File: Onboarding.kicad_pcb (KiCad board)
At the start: 2 copper layers, 40.5 x 26.5 mm, 21 parts, among them J1 Conn_01x02_Female, J2 Conn_01x02_Male, J3 Conn_01x02, J4 Conn_01x02, U1 MC34063A

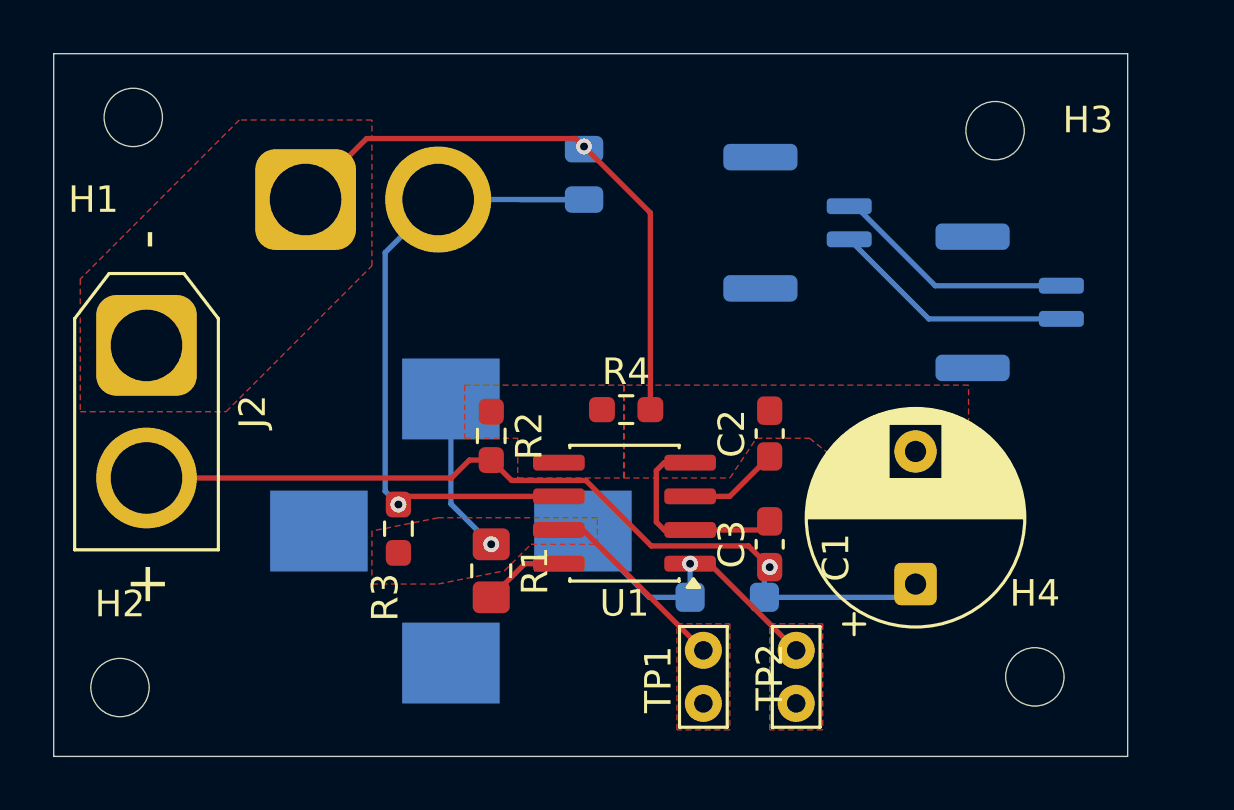
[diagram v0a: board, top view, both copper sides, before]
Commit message: many zones
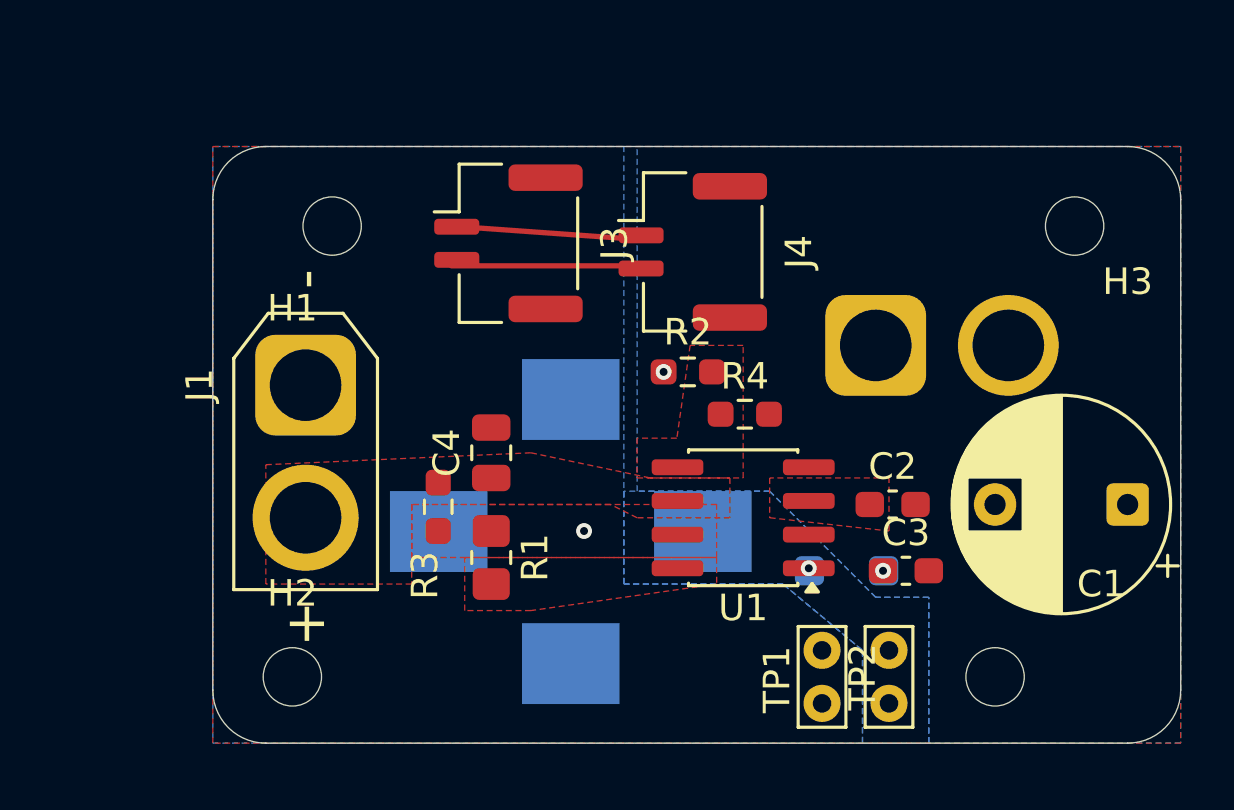
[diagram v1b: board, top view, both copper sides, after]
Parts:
- C4, J1, J3, J4: moved to F.Cu
- J2: moved to B.Cu
- moved J2 27.5 mm to (157.5, 97.0), turned to 0 degrees
- moved J3 19.0 mm to (143.7, 93.2)
- moved C4 11.1 mm to (143.0, 101.0)
- moved H1 8.55 mm to (137.0, 92.5)
- moved C1 8.54 mm to (167.0, 103.0), turned to 180 degrees
- moved R2 7.80 mm to (150.4, 98.0), turned to 180 degrees
- moved J1 7.00 mm to (136.0, 98.5), turned to -90 degrees
- moved H2 6.51 mm to (135.5, 109.5)
- moved C2 5.35 mm to (158.1, 103.0), turned to 0 degrees
- moved C3 5.23 mm to (158.6, 105.5), turned to 0 degrees
- moved H3 4.68 mm to (165.0, 92.5)
- moved D2 4.61 mm to (156.4, 105.5)
- moved L1 4.52 mm to (146.0, 104.0)
- moved R4 4.48 mm to (152.6, 99.6)
- moved U1 4.48 mm to (152.5, 103.5)
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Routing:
- net VCC: track 32.6 -> 0.00 mm, vias 3 -> 4
- net GND: track 31.9 -> 0.00 mm, vias 2 -> 0
- net /V_{in}: track 26.6 -> 0.00 mm, vias 1 -> 0
- net Net-(U1-I_{PK}): track 13.4 -> 0.00 mm
- net Net-(D2-A): track 11.7 -> 0.00 mm
- net /CAN-: track 9.24 -> 0.00 mm
- net /CAN+: track 9.24 -> 0.00 mm
- net Net-(U1-CT): track 3.62 -> 0.00 mm
- net Net-(U1-DC): track 3.08 -> 0.00 mm
- added copper zone on F.Cu, net /V_{in}
- added copper zone on B.Cu, net Net-(D2-A)
- added copper zone on F.Cu, net Net-(U1-CT)
- added copper zone on F.Cu, net Net-(U1-DC)
- added copper zone on B.Cu, net Net-(U1-I_{PK})
- added copper zone on B.Cu, net VCC
- removed copper zone on F.Cu, net Net-(D2-A)
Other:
- board size 40.5 x 26.5 mm -> 36.5 x 22.5 mm
